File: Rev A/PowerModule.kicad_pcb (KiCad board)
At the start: 2 copper layers, 100 x 100 mm, 106 parts, among them J1 NC6-P108-02, J2 NC6-P108-02, J3 1x7 Socket P2.54mm, K1 Relay_SPDT, Q1 IRLZ44N, Q2 IRLZ44N, Q3 IRLZ44N, U1 LM324, U2 LM324, U3 LM7805

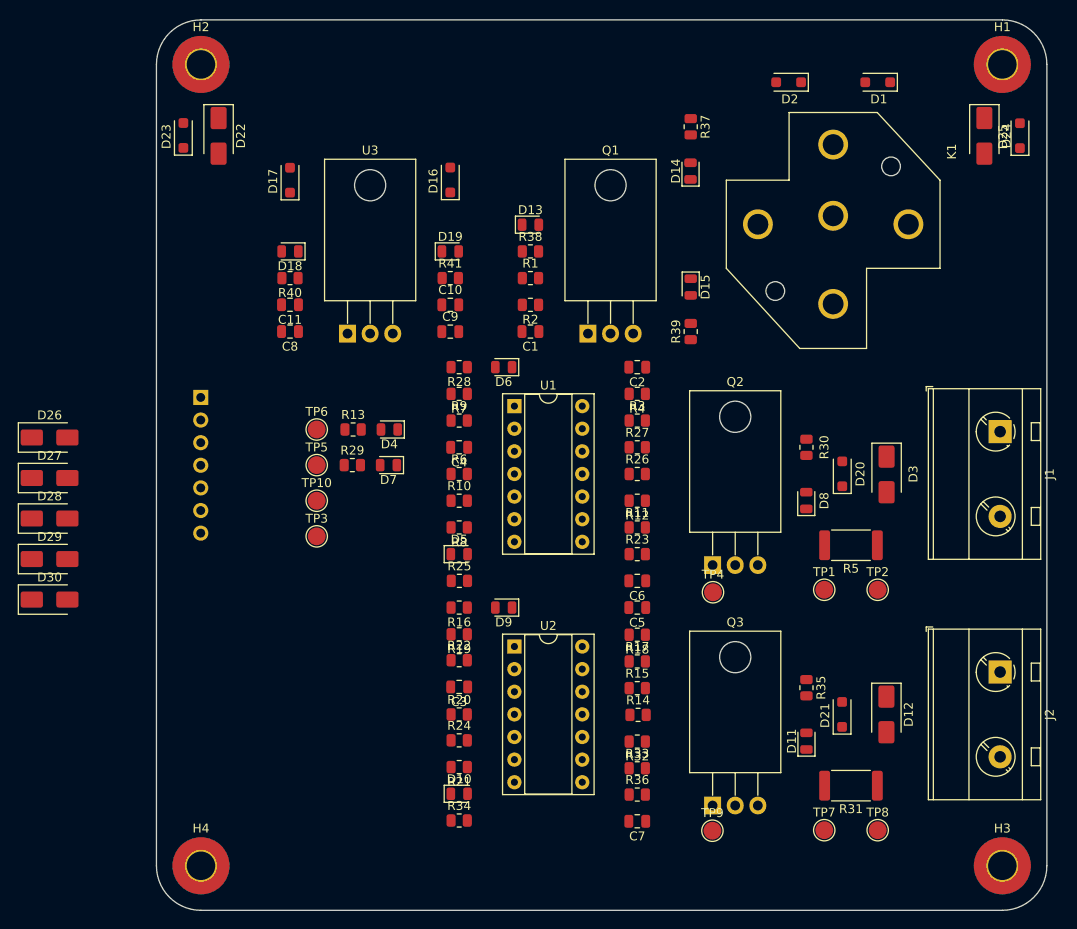
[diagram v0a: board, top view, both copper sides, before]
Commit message: laid out pcb
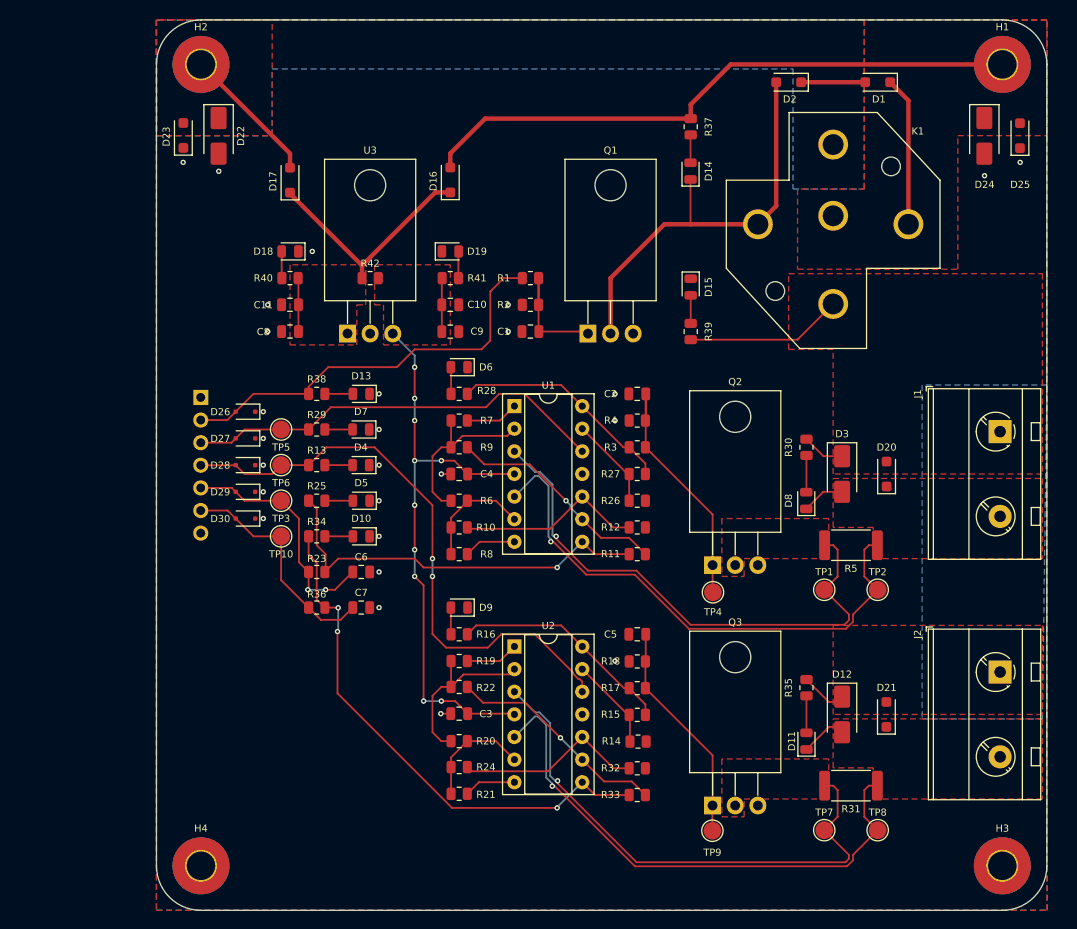
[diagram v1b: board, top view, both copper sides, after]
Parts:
- added R42: 0805,0, Resistor_SMD:R_0805_2012Metric, F.Cu at (121.0, 52.0)
- C6, C7: value 100nF -> 10nF
- D10: value LED Blue -> LED Green
- D26, D27, D28, D29, D30: value SMAJ5.0CA -> PESD3V3L1BA,115; footprint Diode_SMD:D_SMA -> Diode_SMD:D_SOD-323F
- R23, R36: value 100R -> 1K
- moved R36 41.7 mm to (115.0, 89.0), turned to 180 degrees
- moved C7 39.2 mm to (120.0, 89.0), turned to 0 degrees
- moved R23 36.1 mm to (115.0, 85.0), turned to 180 degrees
- moved R34 35.7 mm to (115.0, 81.0)
- moved C6 31.0 mm to (120.0, 85.0), turned to 0 degrees
- moved D10 30.9 mm to (120.0, 81.0), turned to 180 degrees
- moved R38 28.8 mm to (115.0, 65.0)
- moved D13 26.9 mm to (120.0, 65.0), turned to 180 degrees
- moved D30 23.8 mm to (107.0, 79.0), turned to 180 degrees
- moved D29 23.3 mm to (107.0, 76.0), turned to 180 degrees
- moved D28 22.8 mm to (107.0, 73.0), turned to 180 degrees
- moved D27 22.4 mm to (107.0, 70.0), turned to 180 degrees
- moved D26 22.2 mm to (107.0, 67.0), turned to 180 degrees
- moved R25 18.4 mm to (115.0, 77.0)
- moved D5 12.5 mm to (120.0, 77.0), turned to 180 degrees
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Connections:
- net +5VA renamed /OpAmpPWR
- net Net-(D16-K) renamed /VIN_OPA_PWR
- net Net-(R11-Pad2) renamed /ISen1_unfilt
- net Net-(R33-Pad2) renamed /ISen2_unfilt
- C6 pad 1: /CurrentSenseCh2 -> /CurrentSenseCh1
- C7 pad 1: /CurrentSenseCh1 -> /CurrentSenseCh2
- D11 pad 1: /ISense1_P -> /ISense2_P
- D12 pad 2: /ISense1_P -> /ISense2_P
- D20 pad 1: /ISense2_P -> /ISense1_P
- D21 pad 1: /ISense1_P -> /ISense2_P
- D3 pad 2: /ISense2_P -> /ISense1_P
- D8 pad 1: /ISense2_P -> /ISense1_P
- J1 pad 2: /ISense2_P -> /ISense1_P
- J2 pad 2: /ISense1_P -> /ISense2_P
- Q2 pad 2: /ISense2_N -> /ISense1_N
- Q3 pad 2: /ISense1_N -> /ISense2_N
- R13 pad 1: /PWM_Lights1 -> /PWM_Lights2
- R23 pad 2: /CurrentSenseCh2 -> /CurrentSenseCh1
- R29 pad 1: /PWM_Lights2 -> /PWM_Lights1
- R31 pad 1: /ISense1_P -> /ISense2_P
- R31 pad 2: /ISense1_N -> /ISense2_N
- R36 pad 2: /CurrentSenseCh1 -> /CurrentSenseCh2
- R5 pad 1: /ISense2_P -> /ISense1_P
- R5 pad 2: /ISense2_N -> /ISense1_N
- TP1 pad 1: /ISense2_N -> /ISense1_N
- TP10 pad 1: /CurrentSenseCh1 -> /CurrentSenseCh2
- TP2 pad 1: /ISense2_P -> /ISense1_P
- TP3 pad 1: /CurrentSenseCh2 -> /CurrentSenseCh1
- TP5 pad 1: /PWM_Lights2 -> /PWM_Lights1
- TP6 pad 1: /PWM_Lights1 -> /PWM_Lights2
- TP7 pad 1: /ISense1_N -> /ISense2_N
- TP8 pad 1: /ISense1_P -> /ISense2_P
- U1 pad 12: /PWM_Lights2 -> /PWM_Lights1
- U1 pad 3: /ISense2_N -> /ISense1_N
- U1 pad 5: /ISense2_P -> /ISense1_P
- U2 pad 12: /PWM_Lights1 -> /PWM_Lights2
- U2 pad 3: /ISense1_N -> /ISense2_N
- U2 pad 5: /ISense1_P -> /ISense2_P
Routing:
- net /12V_HighPreference: track 0.00 -> 85.4 mm
- net /OpAmpPWR: track 0.00 -> 71.4 mm, vias 0 -> 10
- net /PWM_Lights2: track 0.00 -> 66.3 mm, vias 0 -> 2
- net /ISense1_P: track 0.00 -> 66.3 mm, vias 0 -> 1
- net /ISense2_P: track 0.00 -> 66.3 mm, vias 0 -> 1
- net /ISense1_N: track 0.00 -> 60.7 mm, vias 0 -> 1
- net /ISense2_N: track 0.00 -> 60.5 mm, vias 0 -> 1
- net /ISen2_unfilt: track 0.00 -> 59.8 mm, vias 0 -> 3
- net /PWM_Lights1: track 0.00 -> 47.8 mm
- net Net-(D14-K): track 0.00 -> 47.1 mm
- net /RelaySelectHighPreference: track 0.00 -> 46.4 mm
- net /ISen1_unfilt: track 0.00 -> 45.8 mm, vias 0 -> 1
- net /VIN_OPA_PWR: track 0.00 -> 32.3 mm
- net Net-(Q2-G): track 0.00 -> 28.5 mm
- net /12V_Lights: track 0.00 -> 27.5 mm
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- added copper zone on F.Cu, net /12V_HighPreference
- added copper zone on B.Cu, net /12V_Lights
- added copper zone on F.Cu, net /12V_Lights
- added copper zone on B.Cu, net /12V_LowPreference
- added copper zone on F.Cu, net /12V_LowPreference
- added copper zone on F.Cu, net /ISense1_N
- added copper zone on F.Cu, net /ISense1_P
- added copper zone on F.Cu, net /ISense2_N
- added copper zone on F.Cu, net /ISense2_P
- added copper zone on F.Cu, net /OpAmpPWR
- added copper zone on F.Cu, net /VIN_OPA_PWR
- added copper zone on B.Cu, net GND
- added copper zone on F.Cu, net GND
